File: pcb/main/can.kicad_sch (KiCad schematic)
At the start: 2 parts

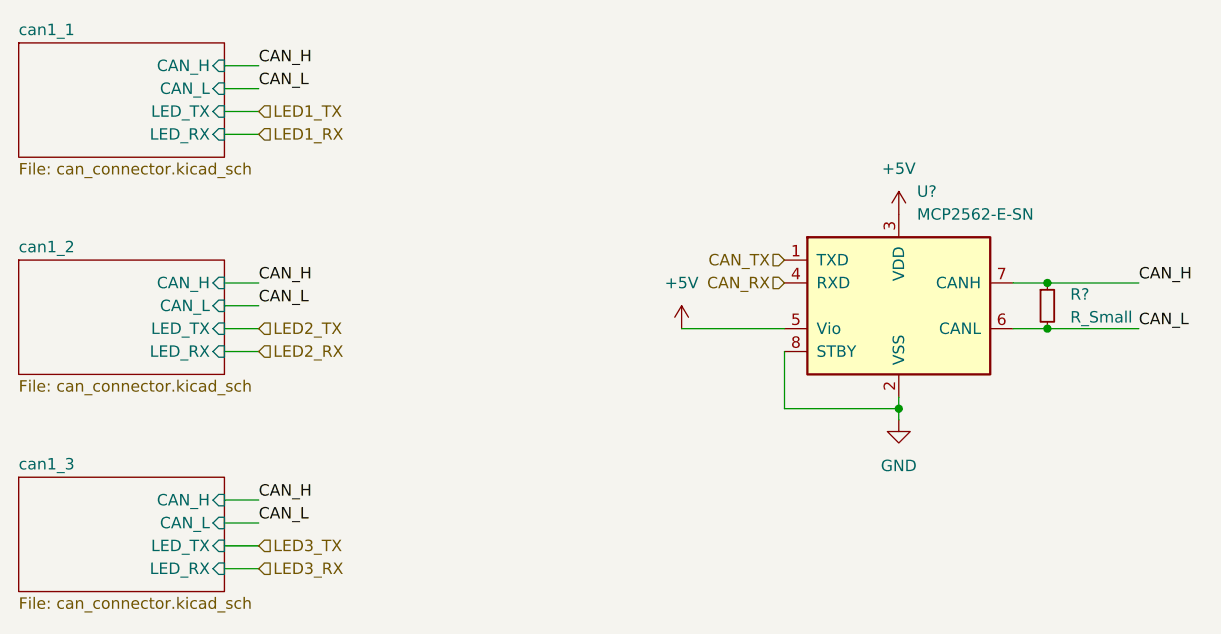
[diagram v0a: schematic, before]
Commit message: chore: add circuit git changes
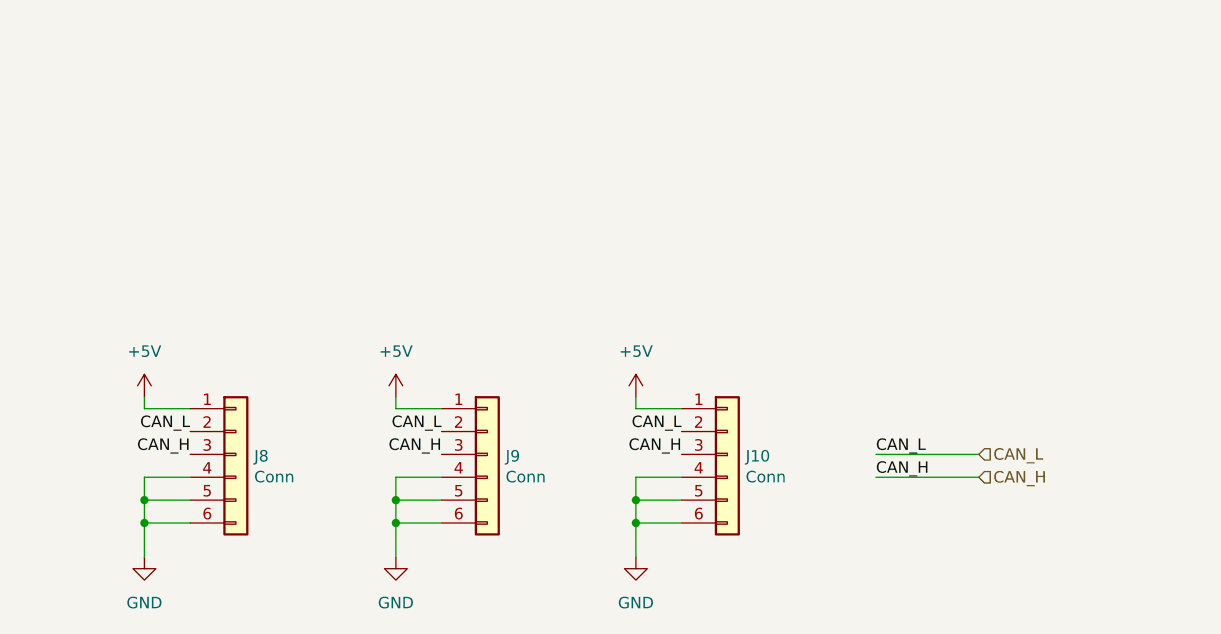
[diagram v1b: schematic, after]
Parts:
- removed R?: R_Small, symbol Device:R_Small
- removed U?: MCP2562-E-SN, Package_SO:SOIC-8_3.9x4.9mm_P1.27mm, symbol Interface_CAN_LIN:MCP2562-E-SN
- added J10, J8, J9: Conn, bldc_lib:21322604YY, symbol Connector_Generic:Conn_01x06
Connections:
- net +5V: now also J10.1 (Pin_1), J8.1 (Pin_1), J9.1 (Pin_1)
- net CAN_H: now also J10.3 (Pin_3), J8.3 (Pin_3), J9.3 (Pin_3)
- net CAN_L: now also J10.2 (Pin_2), J8.2 (Pin_2), J9.2 (Pin_2)
- net GND: now also J10.4 (Pin_4), J10.5 (Pin_5), J10.6 (Pin_6), J8.4 (Pin_4), J8.5 (Pin_5), J8.6 (Pin_6), J9.4 (Pin_4), J9.5 (Pin_5), J9.6 (Pin_6)
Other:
- removed sheet can1_1
- removed sheet can1_2
- removed sheet can1_3
